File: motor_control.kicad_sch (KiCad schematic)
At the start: 7 parts, among them Q3 Q_NMOS_DGS, U3 DRV8870DDA

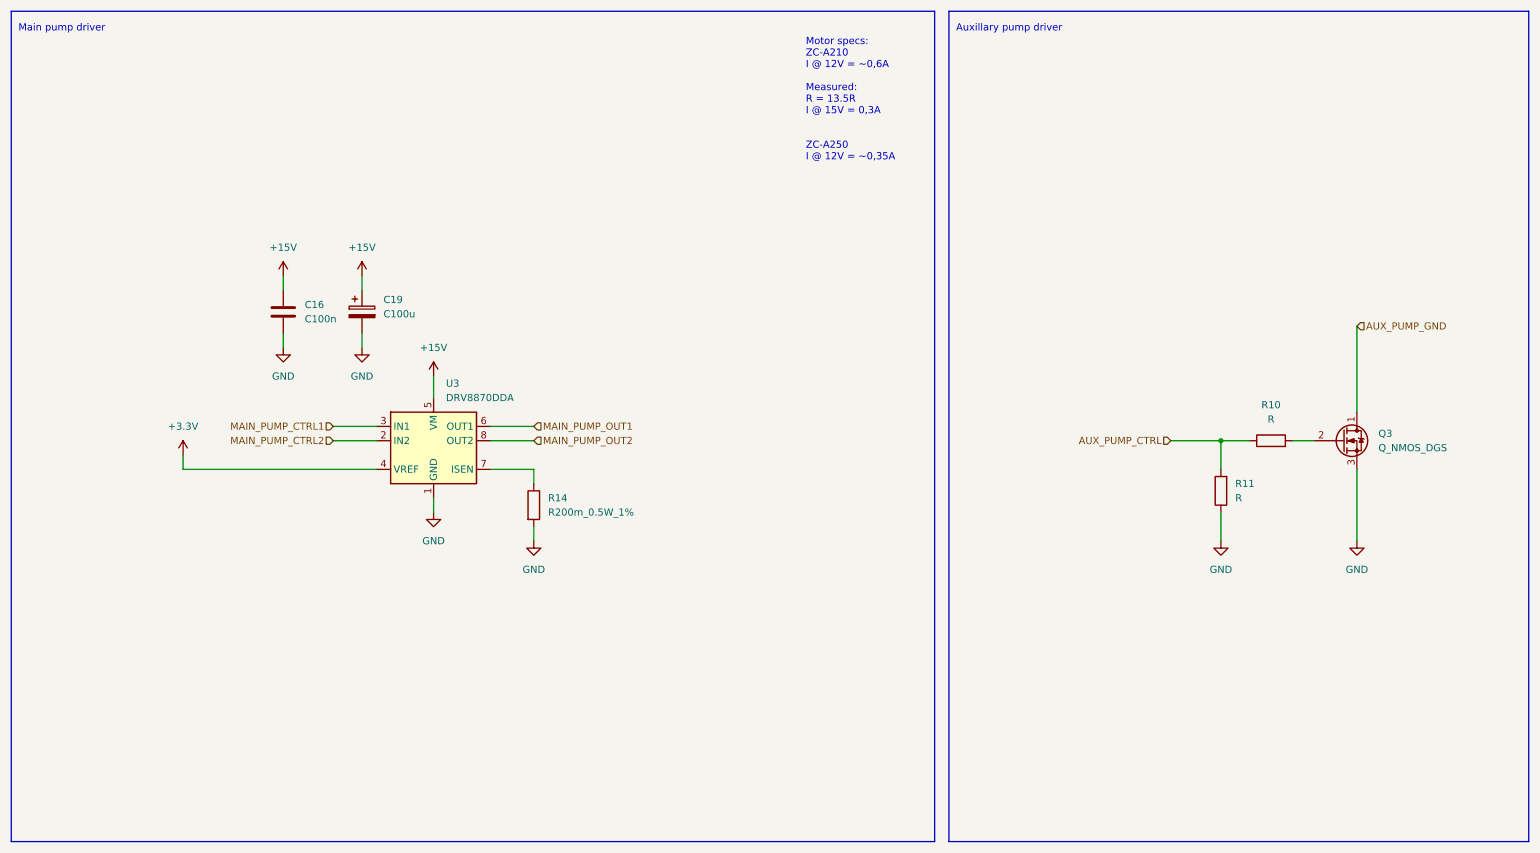
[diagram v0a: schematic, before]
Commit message: Finish first design
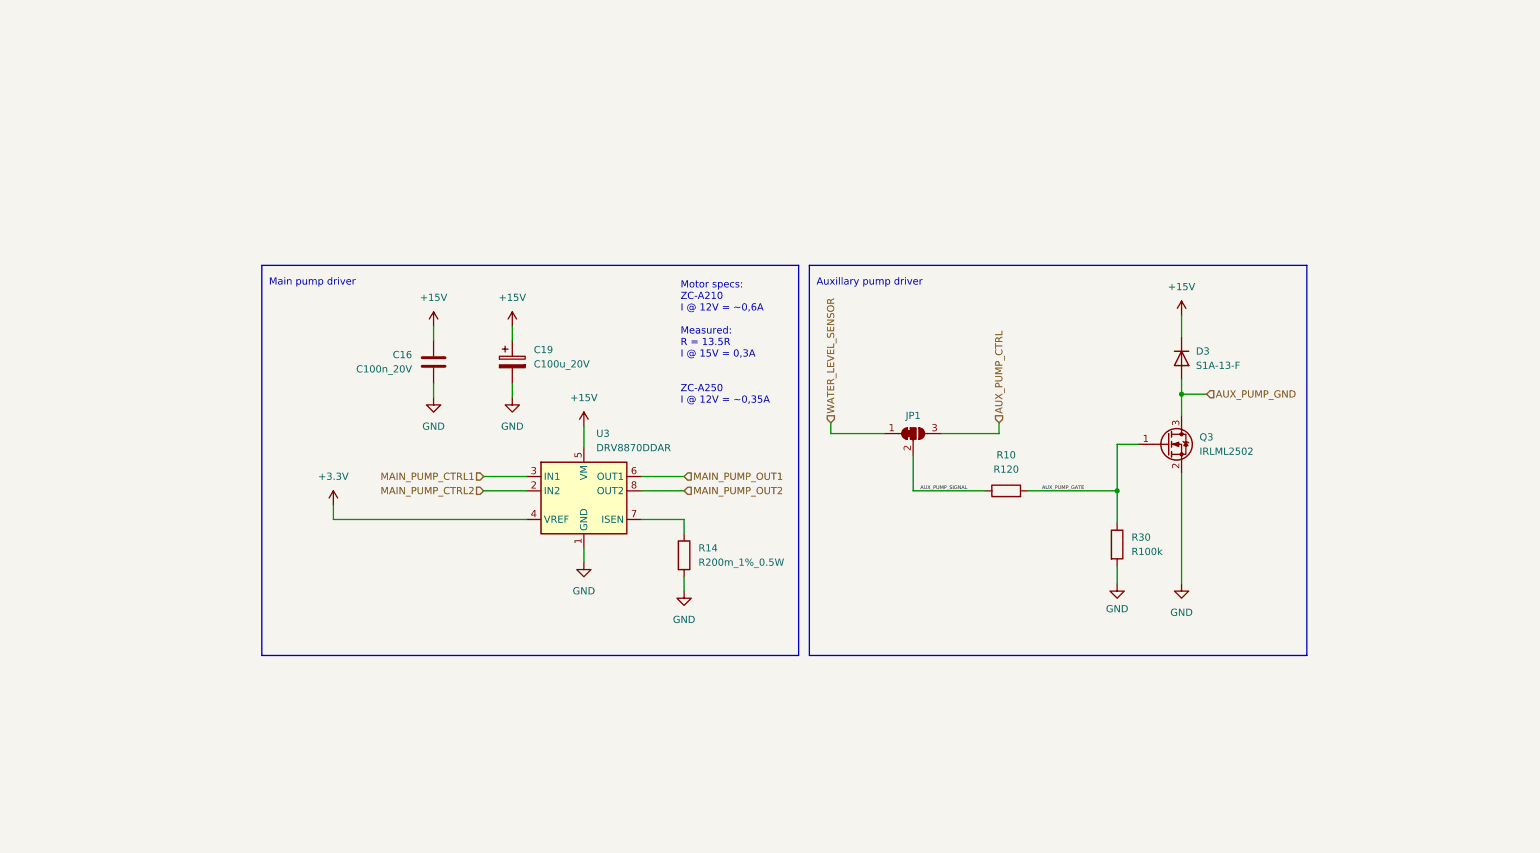
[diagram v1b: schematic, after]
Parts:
- removed Q3: Q_NMOS_DGS, symbol Device:Q_NMOS_DGS
- removed R11: R, symbol Device:R
- added D3: S1A-13-F, Diode_SMD:D_SMA, symbol Device:D
- added JP1: SolderJumper_3_Bridged12, Jumper:SolderJumper-3_P1.3mm_Bridged12_RoundedPad1.0x1.5mm_NumberLabels, symbol Jumper:SolderJumper_3_Bridged12
- added Q3: IRLML2502, Package_TO_SOT_SMD:SOT-23, symbol Device:Q_NMOS_GSD
- added R30: R100k, Resistor_SMD:R_0805_2012Metric, symbol Device:R
- C16: value C100n -> C100n_20V; footprint (none) -> Capacitor_SMD:C_0805_2012Metric; Mouser Part Number (none) -> 187-CL21B104KACNNNC
- C19: value C100u -> C100u_20V; footprint (none) -> Capacitor_SMD:CP_Elec_6.3x5.9; Mouser Part Number (none) -> 647-PCM1D101MCL1GS
- R10: value R -> R120; footprint (none) -> Resistor_SMD:R_0805_2012Metric; Mouser Part Number (none) -> 603-AC0805FR-07120RL
- R14: value R200m_0.5W_1% -> R200m_1%_0.5W; footprint (none) -> Resistor_SMD:R_1206_3216Metric; Mouser Part Number (none) -> 504-MFLA1206R2000FS
- U3: value DRV8870DDA -> DRV8870DDAR; Mouser Part Number (none) -> 595-DRV8870DDAR
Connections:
- net +15V: now also D3.1 (K)
- net AUX_PUMP_CTRL: now also JP1.3 (B); no longer R10.1
- net AUX_PUMP_GND: now also D3.2 (A), Q3.3 (D)
- net GND: now also Q3.2 (S), R30.2
- net AUX_PUMP_GATE: now reaches R10.2
- net AUX_PUMP_GATE: now also Q3.1 (G), R30.1
- new net AUX_PUMP_SIGNAL: JP1.2 (C), R10.1
- new net WATER_LEVEL_SENSOR: JP1.1 (A)
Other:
- moved on the sheet: C16, C19, R10, R14, U3
